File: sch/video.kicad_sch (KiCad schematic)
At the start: 4 parts

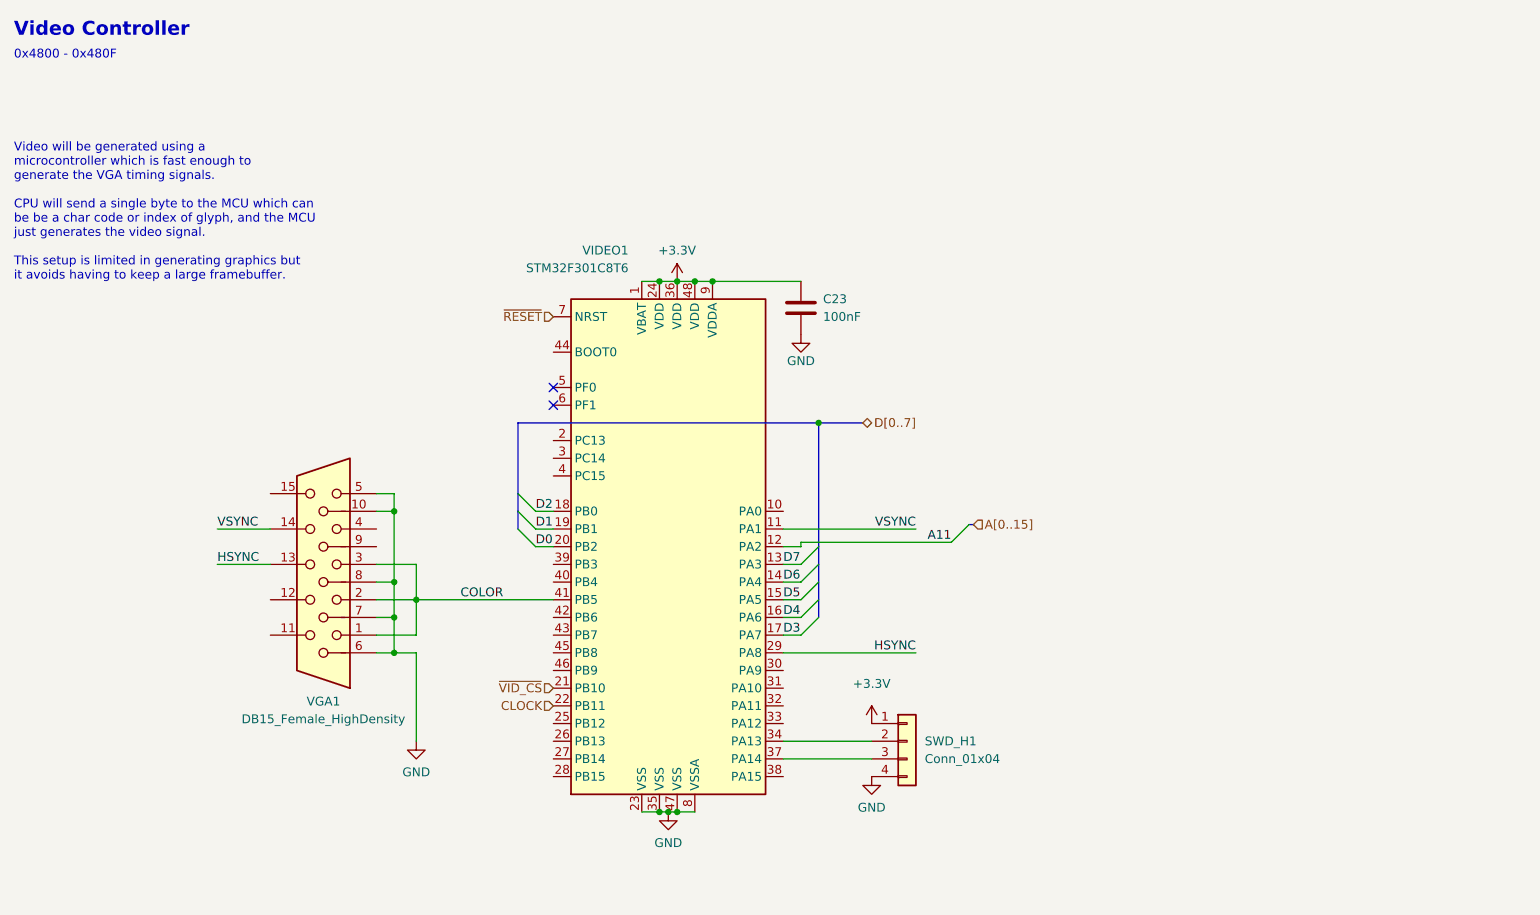
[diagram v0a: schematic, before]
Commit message: Clearances
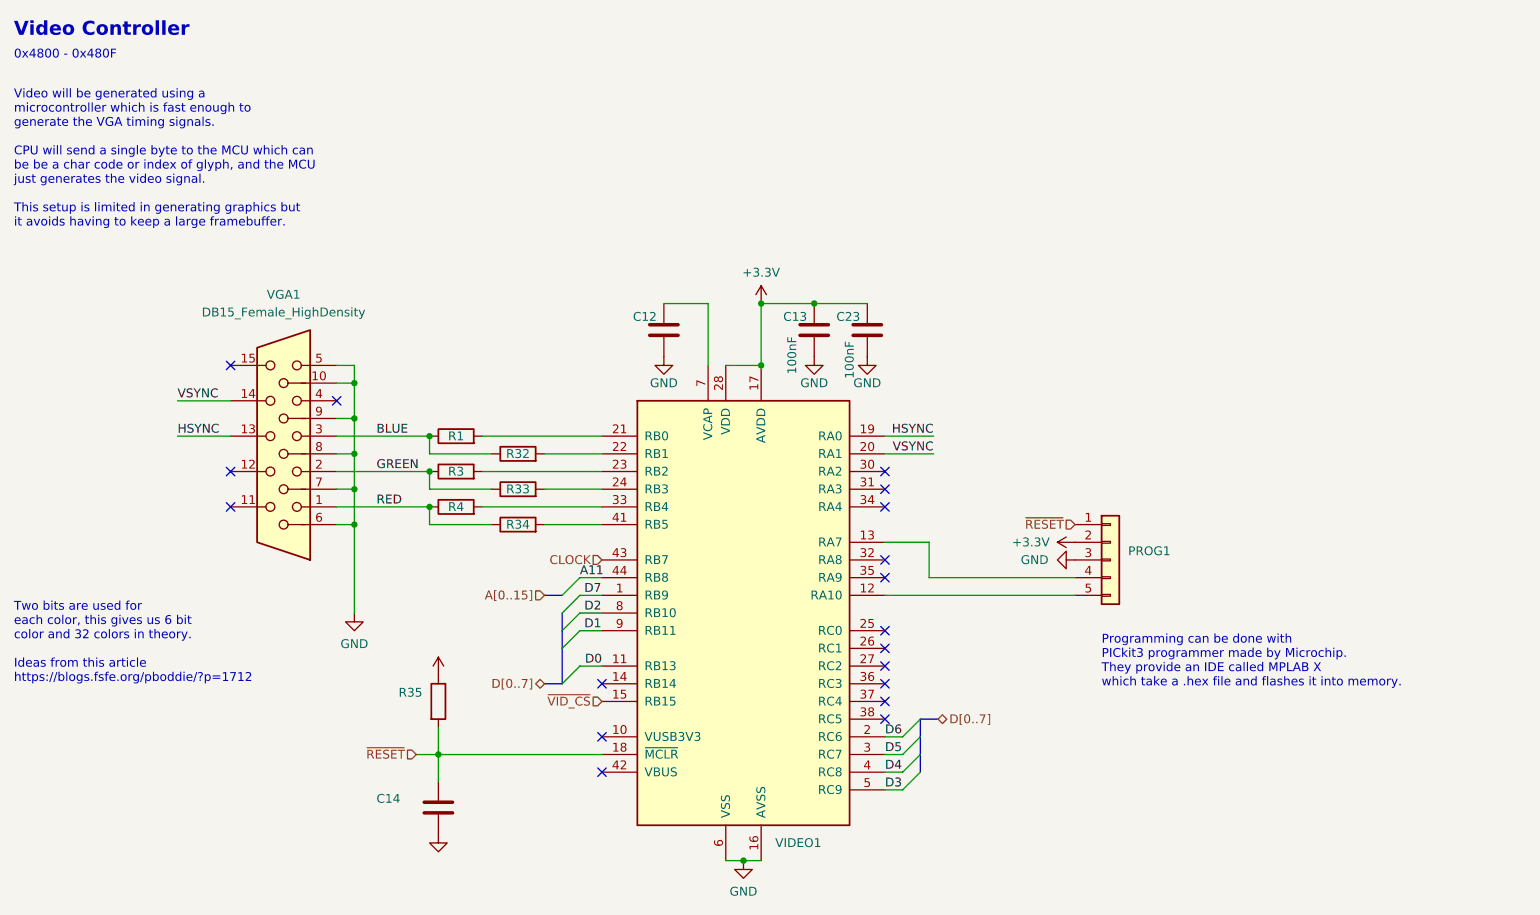
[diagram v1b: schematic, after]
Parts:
- removed VIDEO1: STM32F301C8T6, Package_QFP:TQFP-48_7x7mm_P0.5mm, symbol MCU_ST_STM32F3:STM32F301C6Tx
- added C12: (no value), Capacitor_SMD:C_0805_2012Metric, symbol Device:C
- added C13: 100nF, Capacitor_SMD:C_0805_2012Metric, symbol Device:C
- added C14: (no value), symbol Device:C
- added R1, R3, R32, R33, R34, R35, R4: (no value), symbol Device:R
- added VIDEO1: (no value), symbol MCU_Microchip_PIC32:PIC32MX270F256D-IPT
- PROG1: renamed from SWD_H1; value Conn_01x04 -> (none); footprint Connector_PinHeader_2.00mm:PinHeader_1x04_P2.00mm_Vertical -> (none); symbol Connector_Generic:Conn_01x04 -> Connector_Generic:Conn_01x05
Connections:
- net +3V3: now also PROG1.2 (Pin_2), C13.1, R35.1, VIDEO1.17 (AVDD), VIDEO1.28 (VDD), VIDEO1.40 (VDD); no longer PROG1.1 (Pin_1)
- net A11: now also VIDEO1.44 (RB8)
- net CLOCK: now also VIDEO1.43 (RB7)
- net D0: now also VIDEO1.11 (RB13)
- net D1: now also VIDEO1.9 (RB11)
- net D2: now also VIDEO1.8 (RB10)
- net D3: now also VIDEO1.5 (RC9)
- net D4: now also VIDEO1.4 (RC8)
- net D5: now also VIDEO1.3 (RC7)
- net D6: now also VIDEO1.2 (RC6)
- net D7: now also VIDEO1.1 (RB9)
- net GND: now also PROG1.3 (Pin_3), VGA1.9, C12.2, C13.2, C14.2, VIDEO1.16 (AVSS), VIDEO1.29 (VSS), VIDEO1.39 (VSS), VIDEO1.6 (VSS); no longer PROG1.4 (Pin_4)
- net HSYNC: now also VIDEO1.19 (RA0)
- net VSYNC: now also VIDEO1.20 (RA1)
- net ~{RESET}: now also PROG1.1 (Pin_1), C14.1, R35.2, VIDEO1.18 (~{MCLR})
- net ~{VID_CS}: now also VIDEO1.15 (RB15)
- removed net COLOR: VGA1.1, VGA1.2, VGA1.3
- new net: R3.2, VIDEO1.23 (RB2)
- new net: R32.2, VIDEO1.22 (RB1)
- new net: R34.2, VIDEO1.41 (RB5)
- new net: C12.1, VIDEO1.7 (VCAP)
- new net: R1.2, VIDEO1.21 (RB0)
- new net: PROG1.5 (Pin_5), VIDEO1.12 (RA10)
- new net: PROG1.4 (Pin_4), VIDEO1.13 (RA7)
- new net: R33.2, VIDEO1.24 (RB3)
- new net: R4.2, VIDEO1.33 (RB4)
- new net BLUE: R1.1, R32.1, VGA1.3
- new net GREEN: R3.1, R33.1, VGA1.2
- new net RED: R34.1, R4.1, VGA1.1
- no-connect marks 2 -> 18
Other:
- note added: "Programming can be done with PICkit3 programmer made by Microchip. They provide an IDE called MPLAB X which take a .hex file and flashes it into memory."
- note added: "Two bits are used for each color, this gives us 6 bit color and 32 colors in theory. Ideas from this article https://blogs.fsfe.org/pboddie/?p=1712"
- moved on the sheet: C23, VGA1
